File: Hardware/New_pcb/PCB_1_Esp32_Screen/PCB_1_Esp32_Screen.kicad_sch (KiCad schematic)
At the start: 3 parts, among them J1 Conn_01x12_Pin, J2 Conn_01x07_Pin

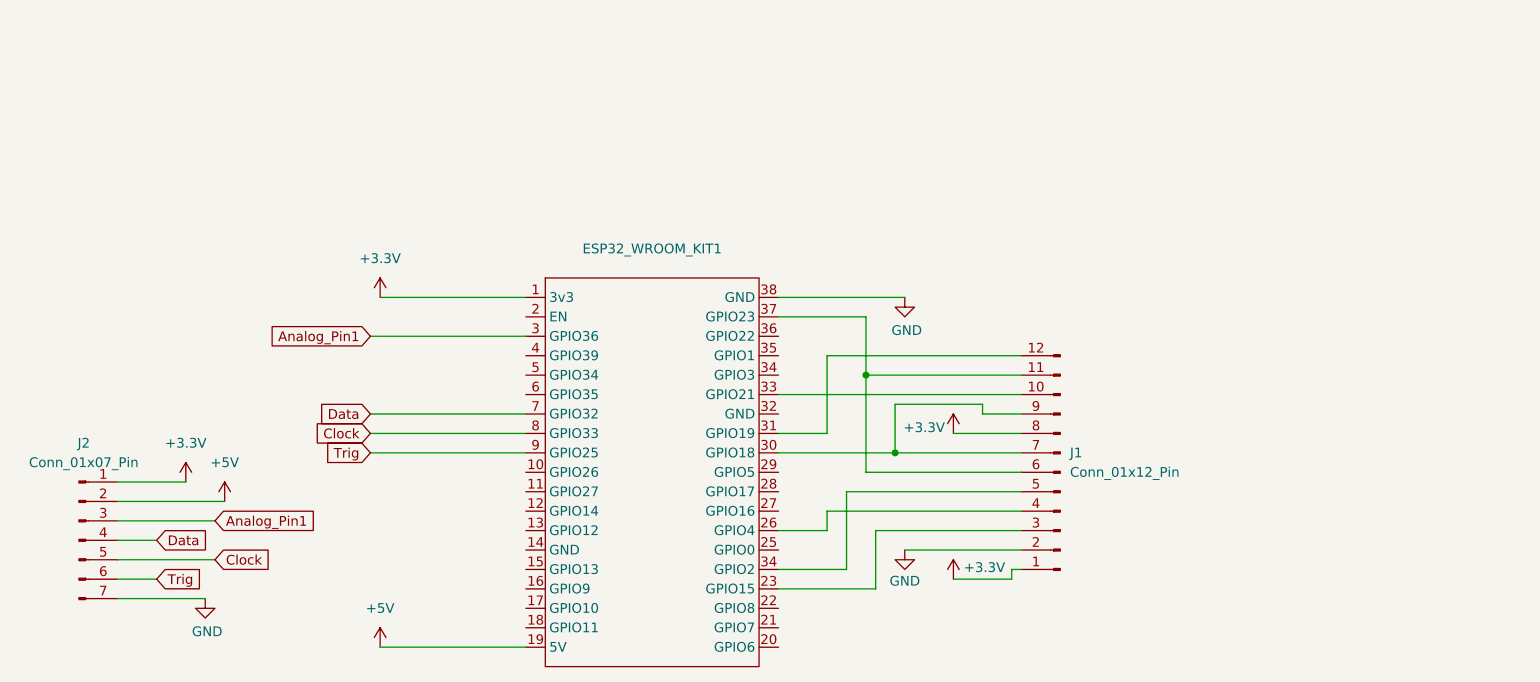
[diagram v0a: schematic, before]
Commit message: pcb amelioration
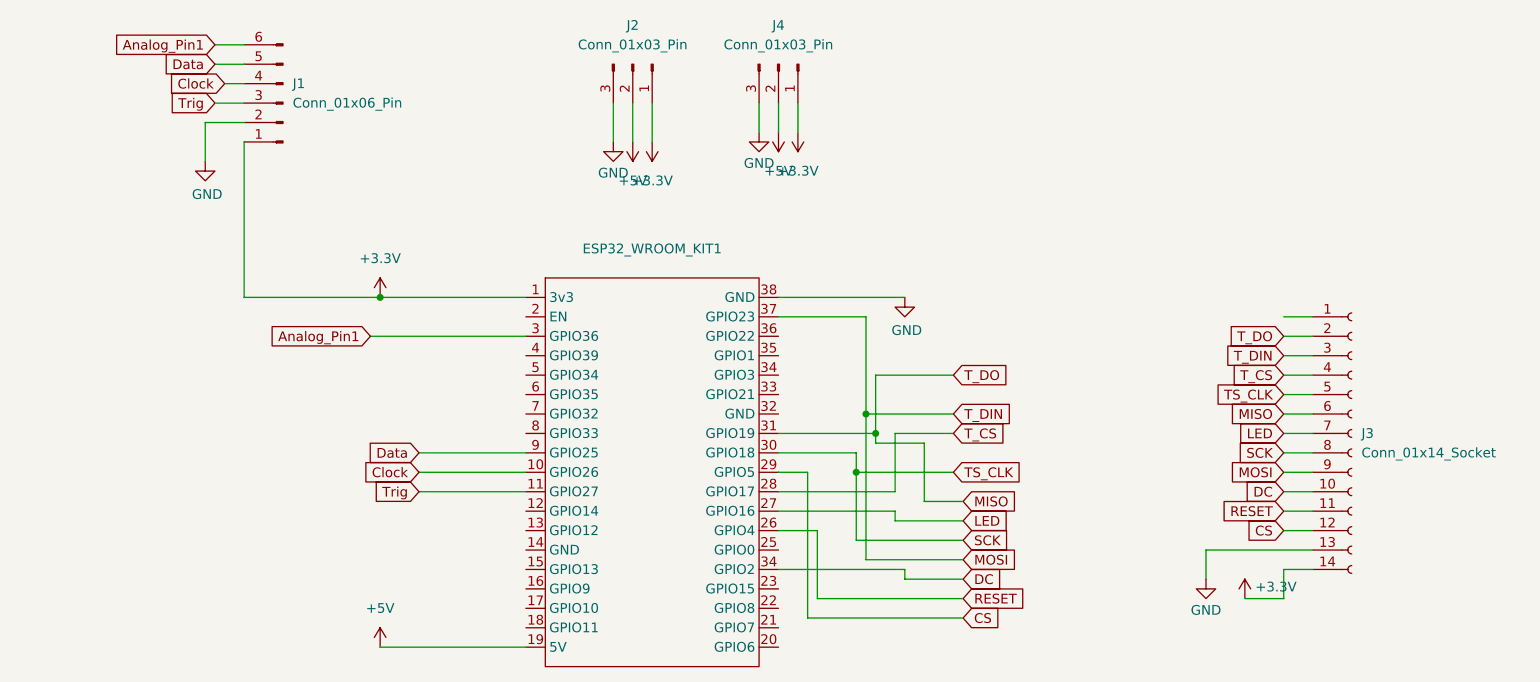
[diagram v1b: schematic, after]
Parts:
- removed J1: Conn_01x12_Pin, Connector_PinHeader_2.54mm:PinHeader_1x12_P2.54mm_Horizontal, symbol Connector:Conn_01x12_Pin
- removed J2: Conn_01x07_Pin, Connector_PinHeader_2.54mm:PinHeader_1x07_P2.54mm_Horizontal, symbol Connector:Conn_01x07_Pin
- added J1: Conn_01x06_Pin, Connector_PinHeader_2.54mm:PinHeader_1x06_P2.54mm_Vertical, symbol Connector:Conn_01x06_Pin
- added J2, J4: Conn_01x03_Pin, Connector_PinHeader_2.54mm:PinHeader_1x03_P2.54mm_Vertical, symbol Connector:Conn_01x03_Pin
- added J3: Conn_01x14_Socket, Connector_PinSocket_2.54mm:PinSocket_1x14_P2.54mm_Vertical, symbol Connector:Conn_01x14_Socket
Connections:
- net +3.3V: now also J1.1 (Pin_1), J2.1 (Pin_1), J3.14 (Pin_14), J4.1 (Pin_1)
- net +5V: now also J2.2 (Pin_2), J4.2 (Pin_2)
- net Analog_Pin1: now also J1.6 (Pin_6)
- net Clock: now also ESP32_WROOM_KIT1.10 (GPIO26), J1.4 (Pin_4); no longer ESP32_WROOM_KIT1.8 (GPIO33)
- net Data: now also ESP32_WROOM_KIT1.9 (GPIO25), J1.5 (Pin_5); no longer ESP32_WROOM_KIT1.7 (GPIO32)
- net GND: now also J1.2 (Pin_2), J2.3 (Pin_3), J3.13 (Pin_13), J4.3 (Pin_3)
- net Trig: now also ESP32_WROOM_KIT1.11 (GPIO27), J1.3 (Pin_3); no longer ESP32_WROOM_KIT1.9 (GPIO25)
- net RESET: now reaches ESP32_WROOM_KIT1.26 (GPIO4)
- net RESET: now also J3.11 (Pin_11)
- net LED: now reaches ESP32_WROOM_KIT1.27 (GPIO16)
- net LED: now also J3.7 (Pin_7)
- net T_CS: now reaches ESP32_WROOM_KIT1.28 (GPIO17)
- net T_CS: now also J3.4 (Pin_4)
- net CS: now reaches ESP32_WROOM_KIT1.29 (GPIO5)
- net CS: now also J3.12 (Pin_12)
- net SCK: now reaches ESP32_WROOM_KIT1.30 (GPIO18)
- net SCK: now also J3.5 (Pin_5), J3.8 (Pin_8)
- net MISO: now reaches ESP32_WROOM_KIT1.31 (GPIO19)
- net MISO: now also J3.2 (Pin_2), J3.6 (Pin_6)
- net DC: now reaches ESP32_WROOM_KIT1.34 (GPIO3)
- net DC: now also J3.10 (Pin_10)
- net MOSI: now reaches ESP32_WROOM_KIT1.37 (GPIO23)
- net MOSI: now also J3.3 (Pin_3), J3.9 (Pin_9)
